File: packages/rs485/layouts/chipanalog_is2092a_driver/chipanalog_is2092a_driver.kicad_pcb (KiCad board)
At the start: 2 copper layers, 7 parts

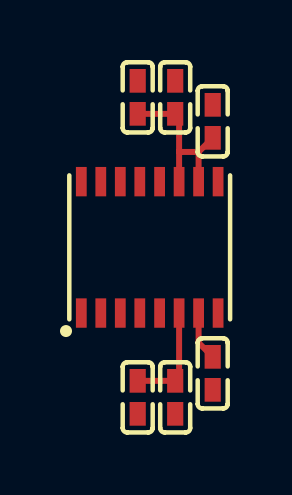
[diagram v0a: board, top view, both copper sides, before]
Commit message: WIP update rs485
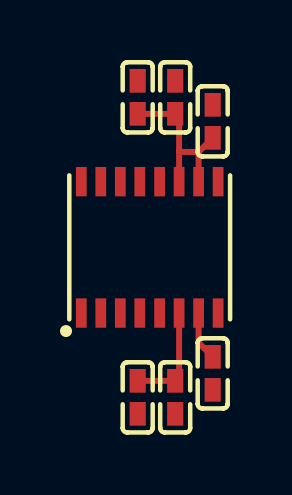
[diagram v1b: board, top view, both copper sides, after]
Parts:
- C1, C2: footprint atopile:C0402-b3ef17 -> Samsung_Electro_Mechanics_CL05A105KA5NQNC:C0402
- C3, C4: value 10µF ±20% 6.3V X5R -> 10µF ±20% 10V X5R; footprint atopile:C0402-b3ef17 -> Samsung_Electro_Mechanics_CL05A106MP5NUNC:C0402
- C5, C6: footprint atopile:C0402-b3ef17 -> Samsung_Electro_Mechanics_CL05B104KO5NNNC:C0402
- U1: footprint atopile:LGA-16_L5.2-W4.7-P0.65-TL_CA-IS2062A-FRANK2-ce0896 -> Chipanalog_CA_IS2092A:LGA-16_L5.2-W4.7-P0.65-TL_CA-IS2062A-FRANK2
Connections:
- C1 pad 2: gnd-1 -> gnd
- C2 pad 2: gnd -> gnd-1
- C3 pad 2: gnd-1 -> gnd
- C4 pad 2: gnd -> gnd-1
- C5 pad 2: gnd-1 -> gnd
- C6 pad 2: gnd -> gnd-1
- U1 pad 12: gnd -> gnd-1
- U1 pad 5: gnd-1 -> gnd
- U1 pad 8: gnd-1 -> gnd
- U1 pad 9: gnd -> gnd-1
